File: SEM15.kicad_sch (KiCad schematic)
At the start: 53 parts, among them J1 Conn_01x04, Q1 AO3401A, Q2 AO3401A, Q3 AO3401A, Q4 AO3401A, SW1 SW_DPST_x2, U1 STC8G1K08-SOP16

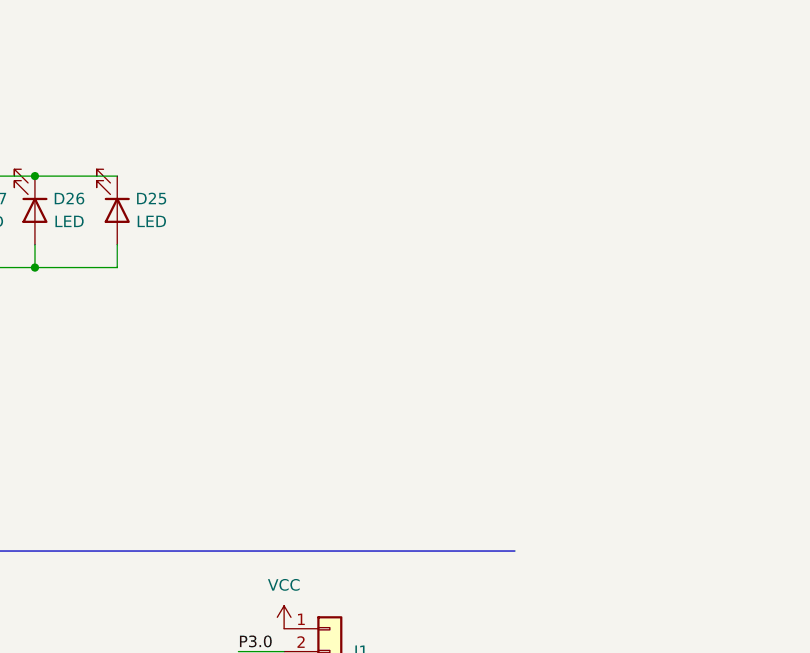
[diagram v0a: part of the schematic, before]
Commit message: rogzitok
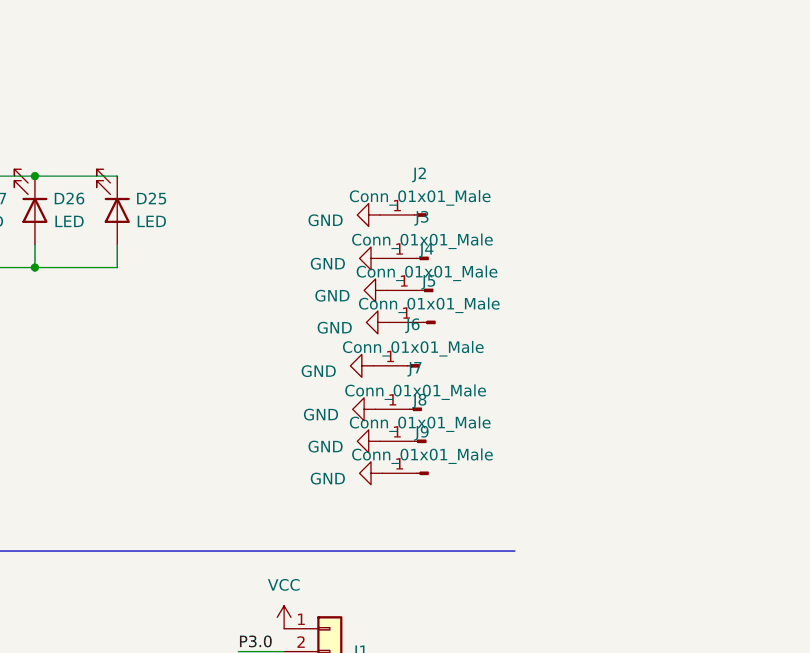
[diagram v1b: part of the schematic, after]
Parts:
- added J2, J3, J4, J5, J6, J7, J8, J9: Conn_01x01_Male, Connector_PinHeader_2.54mm:PinHeader_1x01_P2.54mm_Vertical, symbol Connector:Conn_01x01_Male
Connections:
- net GND: now also J2.1 (Pin_1), J3.1 (Pin_1), J4.1 (Pin_1), J5.1 (Pin_1), J6.1 (Pin_1), J7.1 (Pin_1), J8.1 (Pin_1), J9.1 (Pin_1)
